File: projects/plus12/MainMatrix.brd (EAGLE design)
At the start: 114.3 x 78.1 mm, 43 parts, among them SW1 RSTSWSMD, SW2 TRANSFERPADDY

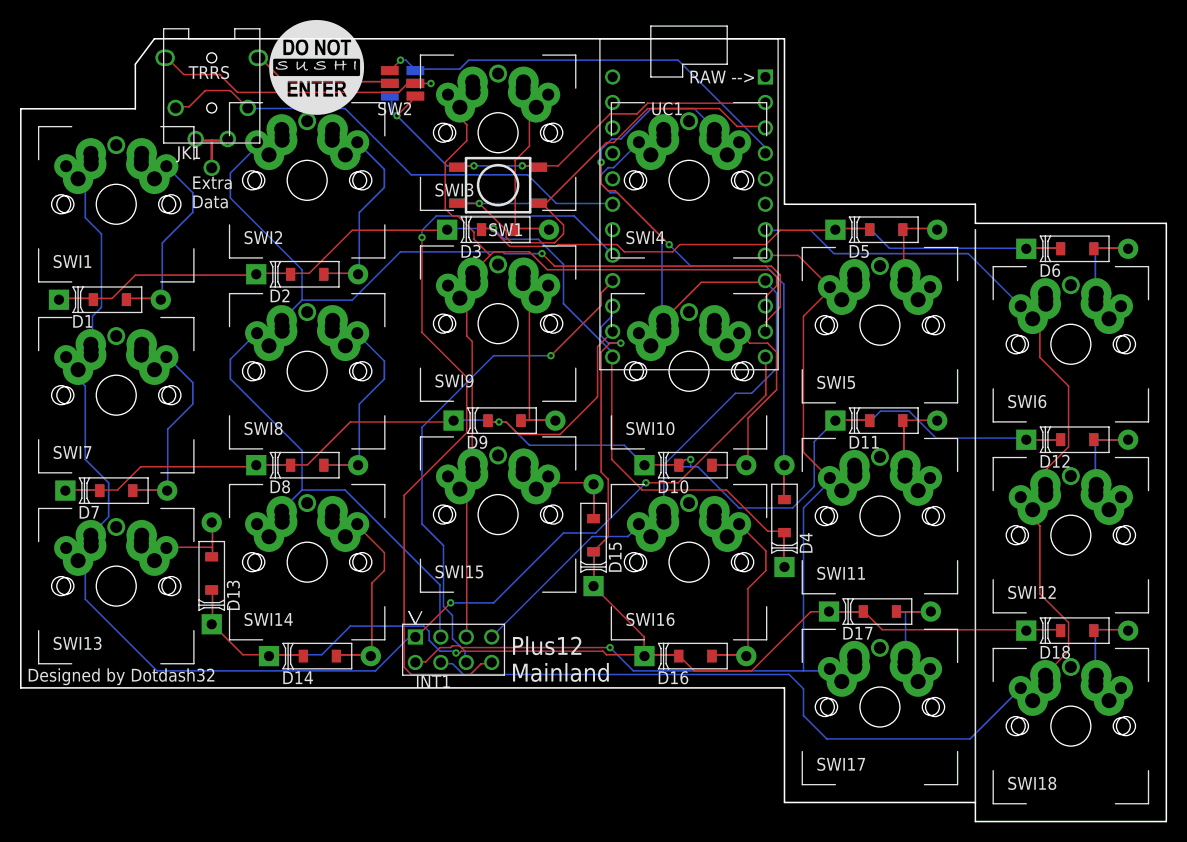
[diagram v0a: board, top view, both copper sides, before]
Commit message: more updates than should be in one commit, lots of work
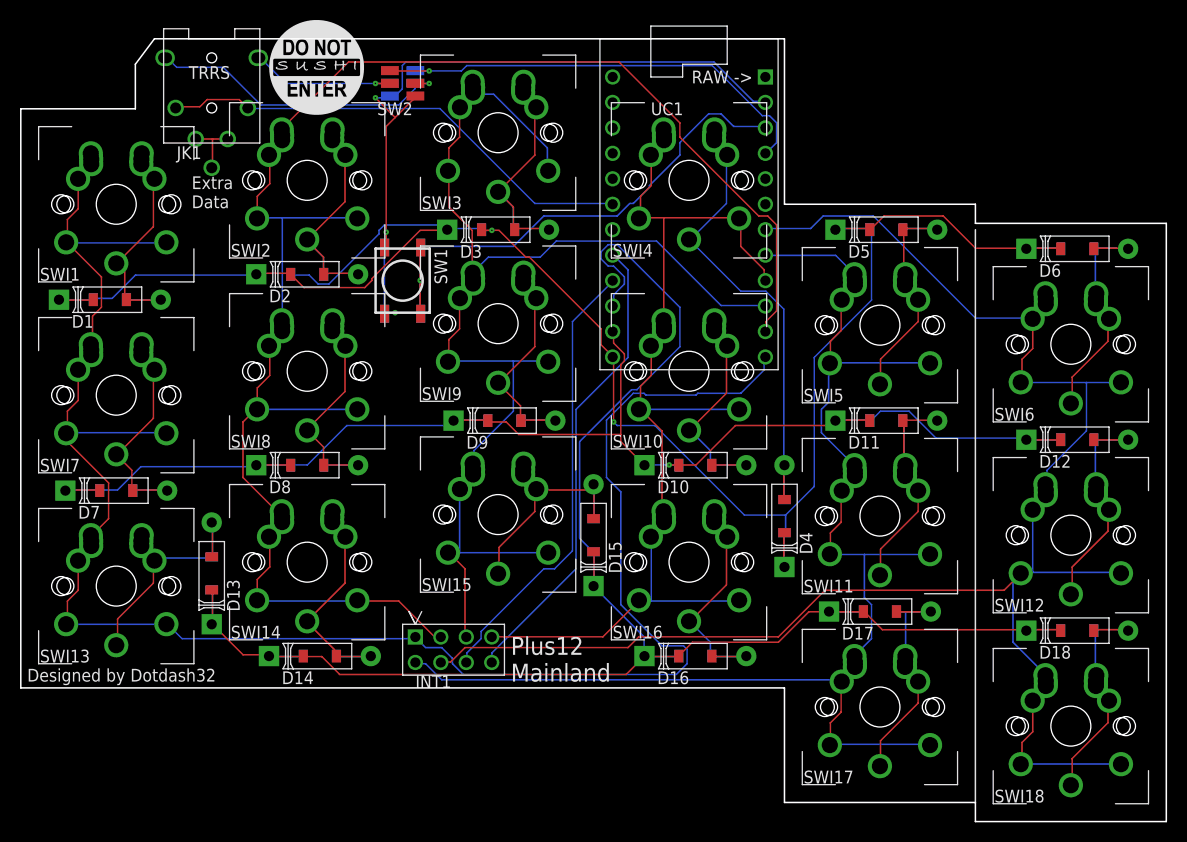
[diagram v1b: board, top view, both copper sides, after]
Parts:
- moved SW1 13.5 mm to (79.4, 94.0), turned to 270 degrees
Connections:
- new net N$36: JK1.3B, JK1.3T, JK1.EXTRA_DATA
- net N$1: now also SWI11.LRLP, SWI17.LRLP, SWI5.LRLP
- net N$10: now also SWI9.RLMID; no longer SWI9.RLP
- net N$11: now also SWI10.RLMID; no longer SWI10.RLP
- net N$12: now also SWI11.RLMID; no longer SWI11.RLP
- net N$13: now also SWI12.RLMID; no longer SWI12.RLP
- net N$14: now also SWI13.RLMID; no longer SWI13.RLP
- net N$15: now also SWI14.RLMID; no longer SWI14.RLP
- net N$16: now also SWI15.RLMID; no longer SWI15.RLP
- net N$17: now also SWI16.RLMID; no longer SWI16.RLP
- net N$18: now also SWI17.RLMID; no longer SWI17.RLP
- net N$19: now also SWI18.RLMID; no longer SWI18.RLP
- net N$2: now also SWI1.RLMID; no longer SWI1.RLP
- net N$23: now also SWI1.LRLP, SWI13.LRLP, SWI7.LRLP
- net N$24: now also SWI14.LRLP, SWI2.LRLP, SWI8.LRLP
- net N$25: now also SWI15.LRLP, SWI3.LRLP, SWI9.LRLP
- net N$26: now also SWI10.LRLP, SWI16.LRLP, SWI4.LRLP
- net N$27: now also SWI12.LRLP, SWI18.LRLP, SWI6.LRLP
- net N$3: now also SWI2.RLMID; no longer SWI2.RLP
- net N$4: now also SWI3.RLMID; no longer SWI3.RLP
- net N$5: now also SWI4.RLMID; no longer SWI4.RLP
- net N$6: now also SWI5.RLMID; no longer SWI5.RLP
- net N$7: now also SWI6.RLMID; no longer SWI6.RLP
- net N$8: now also SWI7.RLMID; no longer SWI7.RLP
- net N$9: now also SWI8.RLMID; no longer SWI8.RLP
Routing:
- net N$23: track 145.6 -> 190.9 mm, vias 2 -> 0
- net N$27: track 149.0 -> 181.3 mm
- net N$33: track 78.8 -> 46.9 mm, vias 1 -> 0
- net N$1: track 109.8 -> 140.7 mm, vias 1 -> 0
- net N$25: track 104.5 -> 132.9 mm
- net N$24: track 142.4 -> 167.5 mm, vias 1 -> 0
- net N$35: track 50.0 -> 73.1 mm
- net N$5: track 71.5 -> 49.8 mm, vias 2 -> 0
- net N$22: track 159.3 -> 174.5 mm, vias 2 -> 0
- net N$31: track 29.3 -> 16.3 mm, vias 0 -> 1
- net N$21: track 150.2 -> 137.4 mm, vias 2 -> 1
- net N$16: track 16.7 -> 28.1 mm
- net N$14: track 16.5 -> 26.7 mm
- net N$20: track 179.3 -> 189.4 mm, vias 1 -> 2
- net N$26: track 100.7 -> 110.4 mm
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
